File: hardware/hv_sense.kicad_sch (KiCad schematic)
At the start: 19 parts, among them IC4 LM393BIDR, U1 PC817

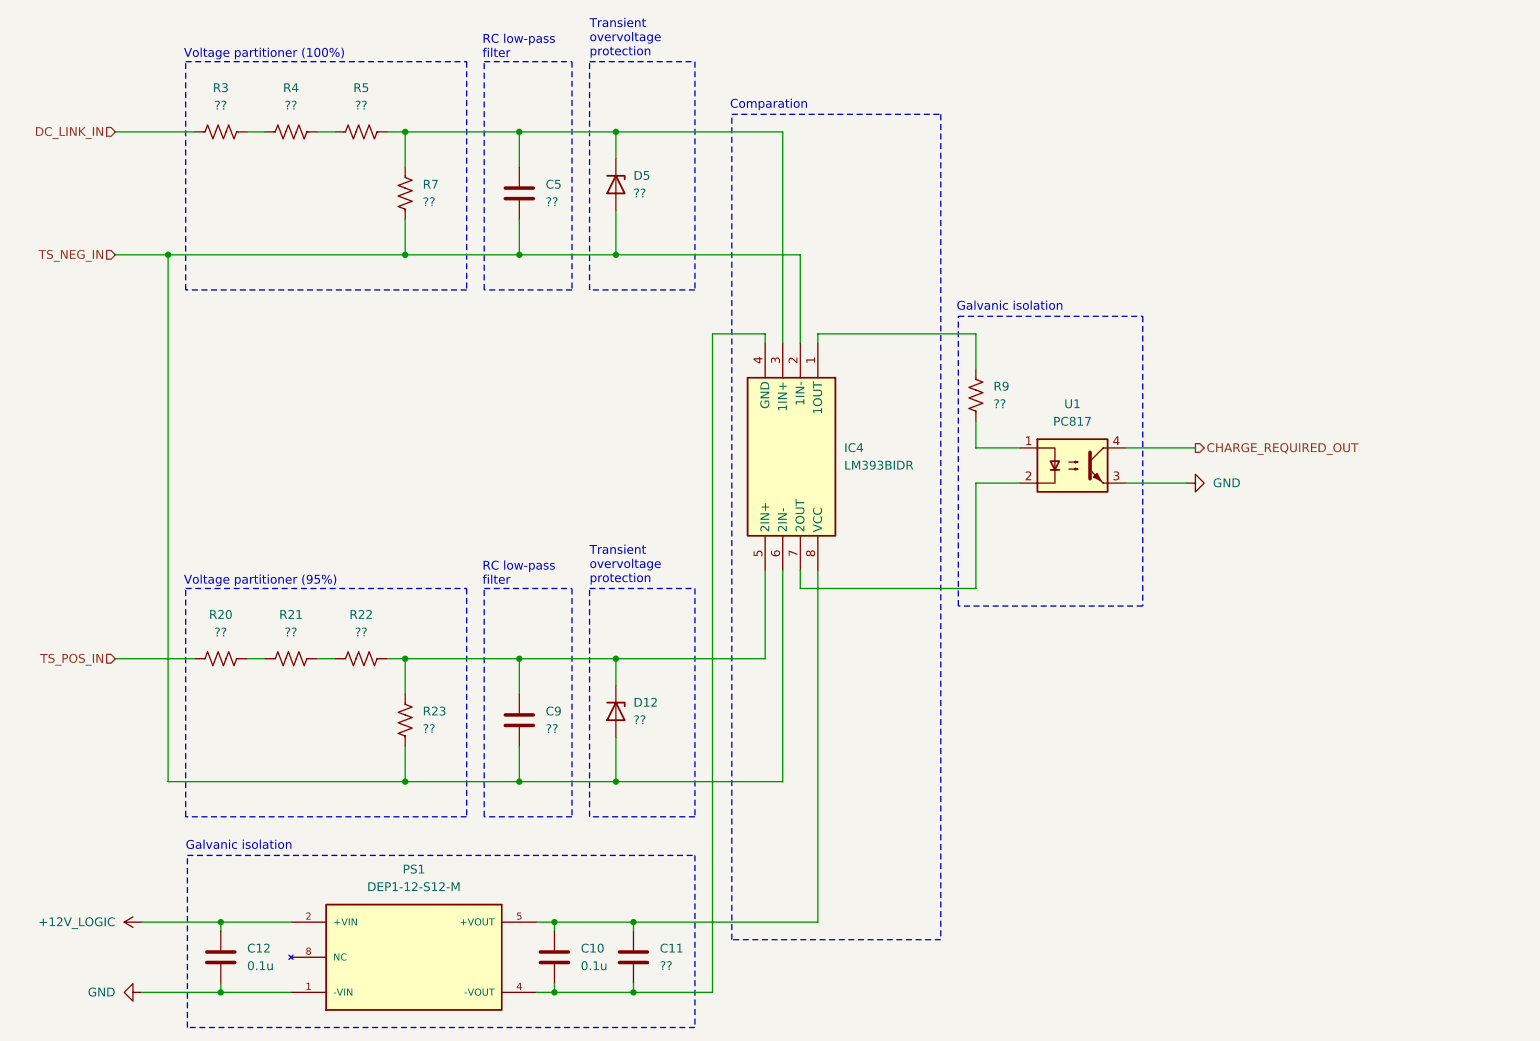
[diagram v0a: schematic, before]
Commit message: start power supply and logic sizing
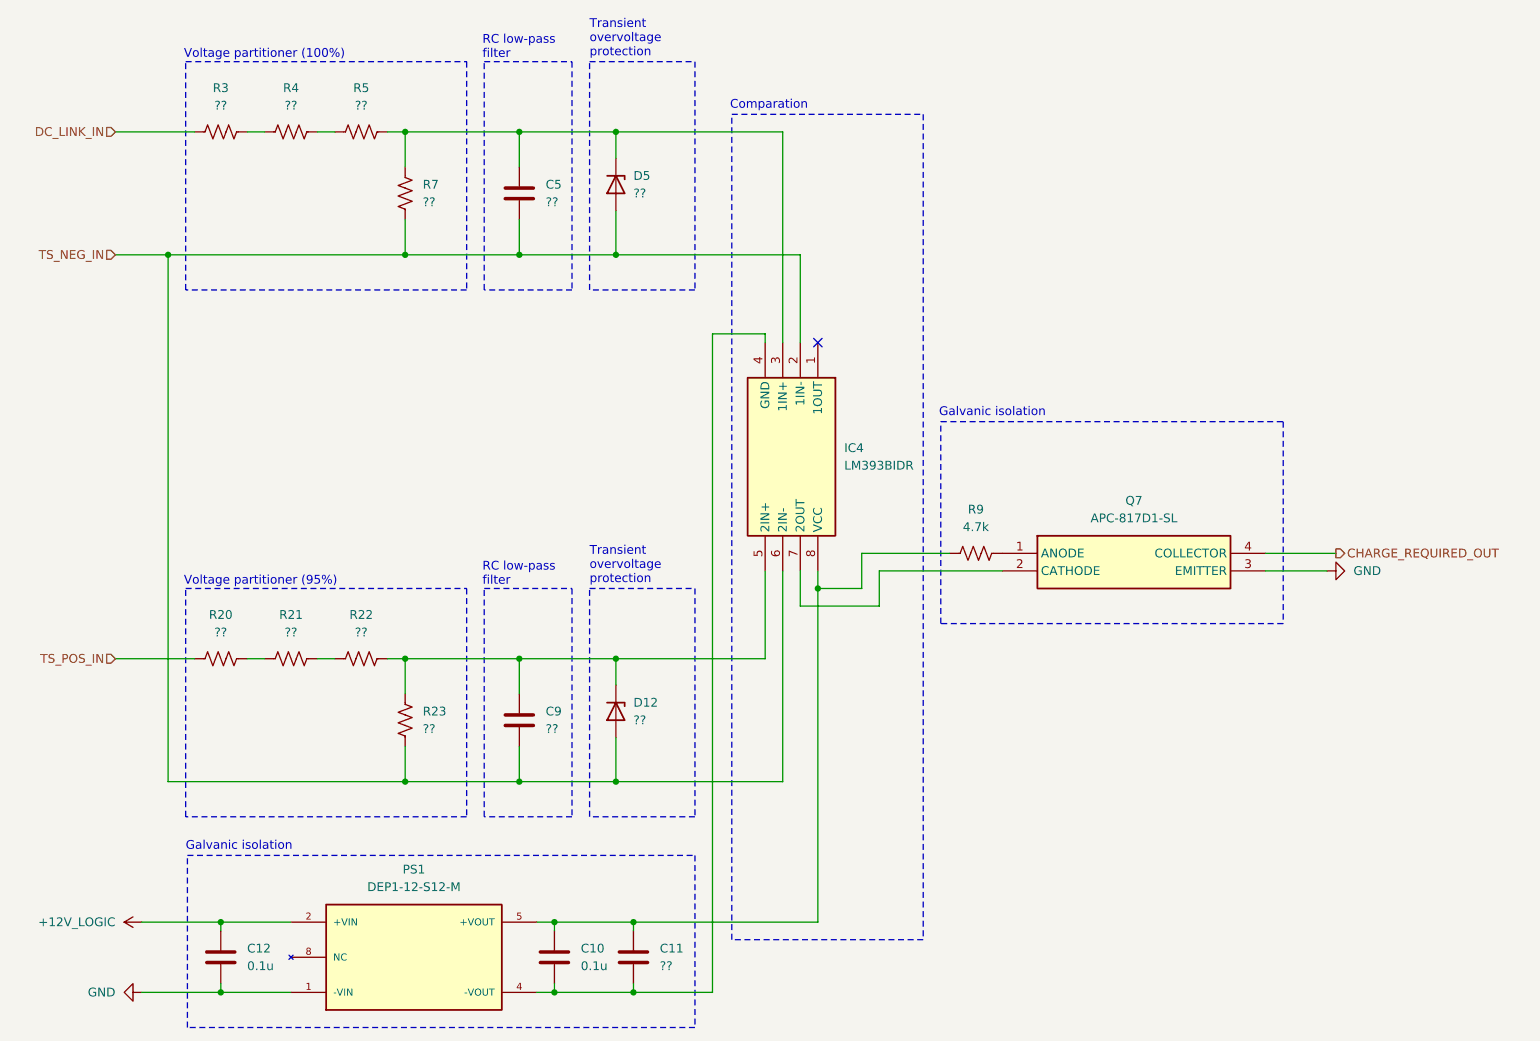
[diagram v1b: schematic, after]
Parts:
- removed U1: PC817, Package_DIP:DIP-4_W7.62mm, symbol Isolator:PC817
- added Q7: APC-817D1-SL, APC817D1SL, symbol Libary_Loader:APC-817D1-SL
- IC4: footprint SOIC127P600X175-8N -> Library_Loader:SOIC127P600X175-8N
- PS1: footprint DEP1-12-S12-M:CONV_DEP1-12-S12-M -> DEP1-12-S12-M:DEP1-12-S12-M
- R9: value ?? -> 4.7k
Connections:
- net CHARGE_REQUIRED_OUT: now also Q7.4 (COLLECTOR)
- net GND: now also Q7.3 (EMITTER)
- net at R9.2: now also Q7.1 (ANODE)
- net at IC4.7 (2OUT): now also Q7.2 (CATHODE)
- net at C10.1, C11.1, IC4.8 (VCC)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: now also R9.1
- net at IC4.1 (1OUT): no longer R9.1
- no-connect marks 0 -> 1
